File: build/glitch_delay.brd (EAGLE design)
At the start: 101.3 x 58.1 mm, 48 parts

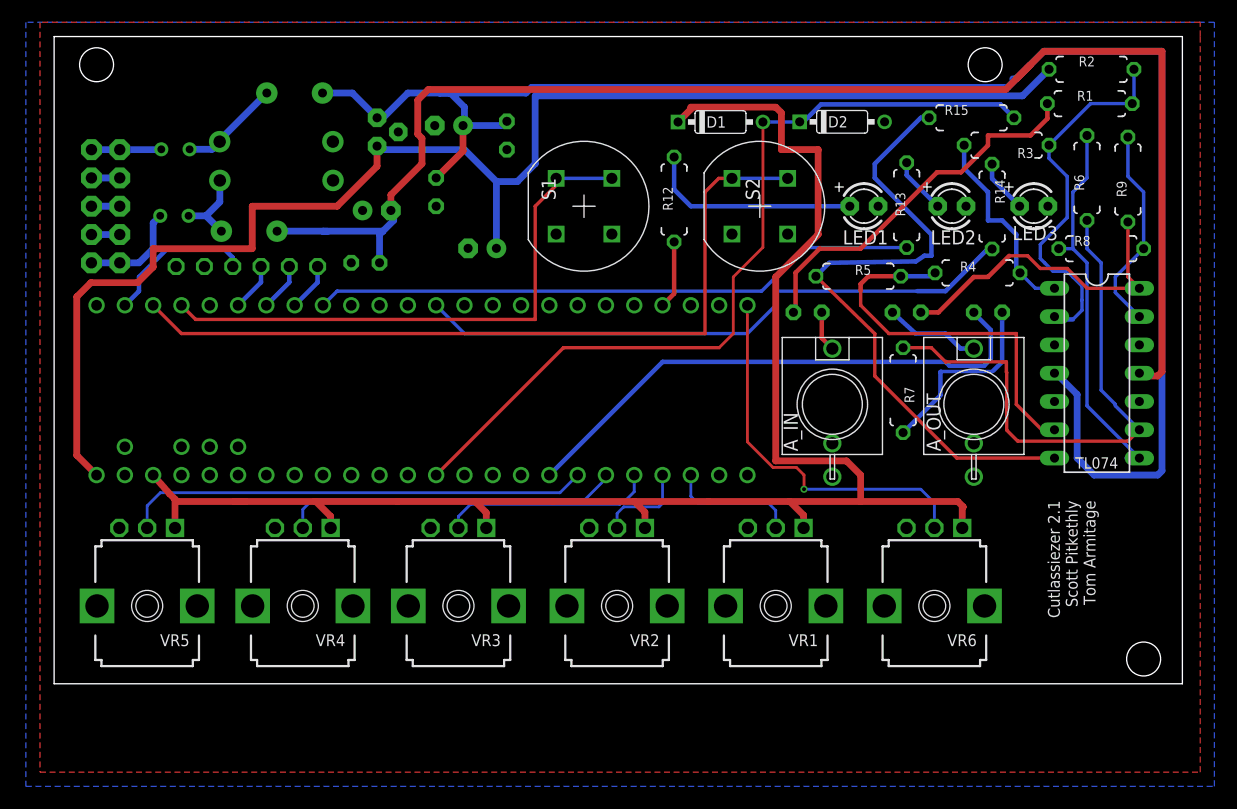
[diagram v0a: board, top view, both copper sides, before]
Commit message: Lots of board tidying.
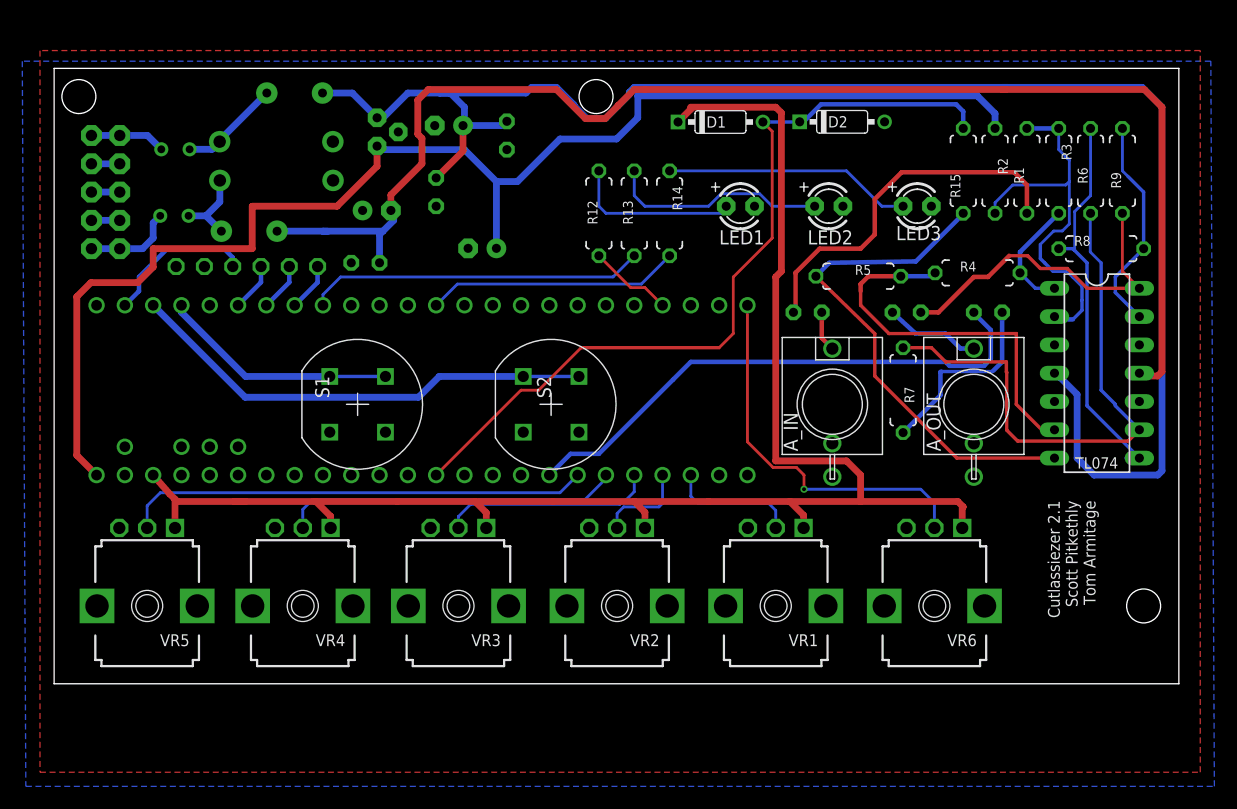
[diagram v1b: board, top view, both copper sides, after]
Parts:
- moved R14 29.0 mm to (55.2, 60.3)
- moved S1 27.0 mm to (27.2, 43.2)
- moved S2 25.8 mm to (44.6, 43.2)
- moved R13 24.5 mm to (52.1, 60.3)
- moved R2 12.6 mm to (84.5, 64.1), turned to 270 degrees
- moved LED1 11.1 mm to (61.6, 61.0)
- moved LED2 11.0 mm to (69.5, 61.0)
- moved LED3 10.5 mm to (77.5, 61.0)
- moved R1 8.27 mm to (87.3, 64.1), turned to 90 degrees
- moved R12 6.87 mm to (48.9, 60.3)
- moved R3 5.22 mm to (90.2, 64.1), turned to 270 degrees
- moved R15 4.82 mm to (81.6, 64.1), turned to 90 degrees
- moved SV1 1.27 mm to (4.62, 62.2)
- moved R9 0.92 mm to (95.9, 64.1)
- moved R6 0.71 mm to (93.0, 64.1)
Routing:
- net N$27: track 54.8 -> 22.8 mm
- net N$20: track 50.7 -> 21.3 mm
- net N$25: track 71.2 -> 42.4 mm
- net N$26: track 54.5 -> 30.3 mm
- net N$23: track 4.81 -> 22.3 mm
- net N$19: track 5.06 -> 19.7 mm
- net N$8: track 58.3 -> 45.9 mm
- net N$4: track 17.9 -> 10.5 mm
- net 5V: track 128.9 -> 122.7 mm
- net -12V: track 128.0 -> 122.9 mm
- net 3.3V: track 147.6 -> 143.0 mm
- net N$9: track 19.3 -> 15.3 mm
- net +12V: track 148.1 -> 145.0 mm
- net A0: track 76.1 -> 73.5 mm
- net N$17: track 6.12 -> 7.56 mm
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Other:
- board size 101.3 x 58.1 mm -> 101 x 55.2 mm
